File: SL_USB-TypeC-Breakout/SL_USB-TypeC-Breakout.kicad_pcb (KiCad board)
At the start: 2 copper layers, 17 x 20 mm, 10 parts, among them J0 USB_C_Receptacle_USB2.0, J1 Conn_01x06, J2 Conn_01x02, J3 Conn_01x01, J4 Conn_01x01

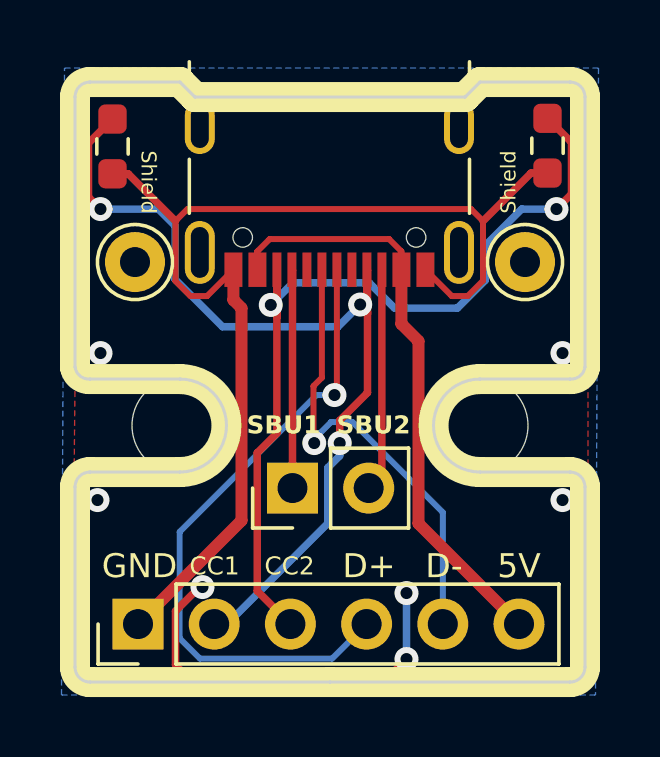
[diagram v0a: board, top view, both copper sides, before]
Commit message: WIP
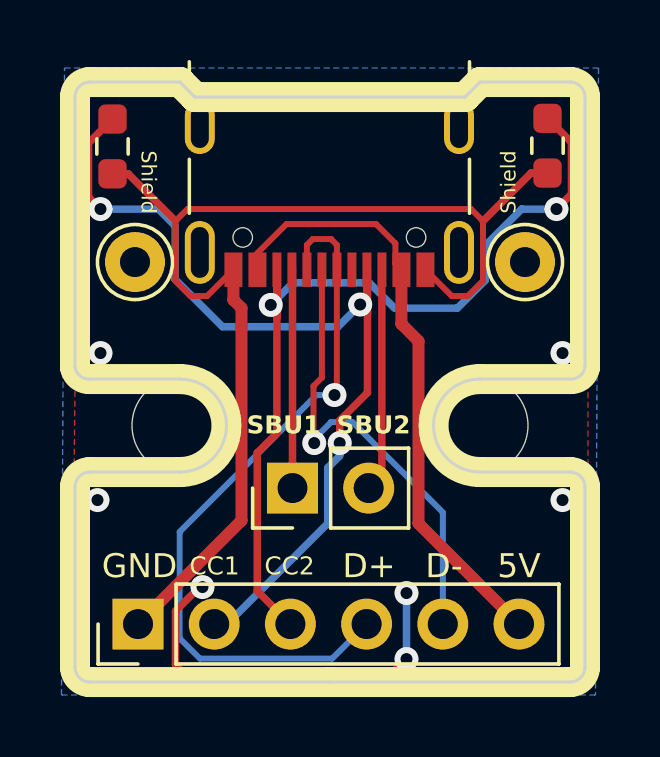
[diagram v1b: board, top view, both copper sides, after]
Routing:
- net /D+: track 21.8 -> 24.6 mm
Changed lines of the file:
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@@
     (effects (font (size 0.8 0.8) (thickness 0.15)))
   )
-  (segment (start 101.23 55.110844) (end 101.23 55.72125) (width 0.2) (layer "F.Cu") (net 1))
+  (segment (start 96.420422 55.711672) (end 96.420422 55.179578) (width 0.2) (layer "F.Cu") (net 1))
   (segment (start 101.23 57.53) (end 101.23 55.72125) (width 0.4) (layer "F.Cu") (net 1))
+  (segment (start 101.03 55.52125) (end 101.23 55.72125) (width 0.2) (layer "F.Cu") (net 1))
+  (segment (start 100.38375 54.2) (end 101.03 54.84625) (width 0.2) (layer "F.Cu") (net 1))
+  (segment (start 97.4 54.2) (end 100.38375 54.2) (width 0.2) (layer "F.Cu") (net 1))
   (segment (start 101.8 58.1) (end 101.23 57.53) (width 0.4) (layer "F.Cu") (net 1))
-  (segment (start 100.819156 54.7) (end 101.23 55.110844) (width 0.2) (layer "F.Cu") (net 1))
+  (segment (start 96.420422 55.179578) (end 97.4 54.2) (width 0.2) (layer "F.Cu") (net 1))
   (segment (start 96.43 55.72125) (end 96.420422 55.711672) (width 0.2) (layer "F.Cu") (net 1))
   (segment (start 101.8 64.18375) (end 101.8 58.1) (width 0.4) (layer "F.Cu") (net 1))
+  (segment (start 101.03 54.84625) (end 101.03 55.52125) (width 0.2) (layer "F.Cu") (net 1))
   (segment (start 105.15 67.53375) (end 101.8 64.18375) (width 0.4) (layer "F.Cu") (net 1))
-  (segment (start 96.420422 55.711672) (end 96.420422 55.120422) (width 0.2) (layer "F.Cu") (net 1))
-  (segment (start 96.420422 55.120422) (end 96.840844 54.7) (width 0.2) (layer "F.Cu") (net 1))
-  (segment (start 96.840844 54.7) (end 100.819156 54.7) (width 0.2) (layer "F.Cu") (net 1))
+  (segment (start 98.27625 54.7) (end 98.88375 54.7) (width 0.2) (layer "F.Cu") (net 2))
   (segment (start 99.08 59.818982) (end 98.9995 59.899482) (width 0.2) (layer "F.Cu") (net 2))
+  (segment (start 99.08 54.89625) (end 99.08 55.72125) (width 0.2) (layer "F.Cu") (net 2))
+  (segment (start 98.08 55.72125) (end 98.08 54.89625) (width 0.2) (layer "F.Cu") (net 2))
   (segment (start 99.08 55.72125) (end 99.08 59.818982) (width 0.2) (layer "F.Cu") (net 2))
+  (segment (start 98.08 54.89625) (end 98.27625 54.7) (width 0.2) (layer "F.Cu") (net 2))
+  (segment (start 98.88375 54.7) (end 99.08 54.89625) (width 0.2) (layer "F.Cu") (net 2))
   (via (at 98.9995 59.899482) (size 0.8) (drill 0.4) (layers "F.Cu" "B.Cu") (free) (net 2))
   (segment (start 98.400518 59.899482) (end 93.84 64.46) (width 0.2) (layer "B.Cu") (net 2))
